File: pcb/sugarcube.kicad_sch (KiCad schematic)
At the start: 0 parts

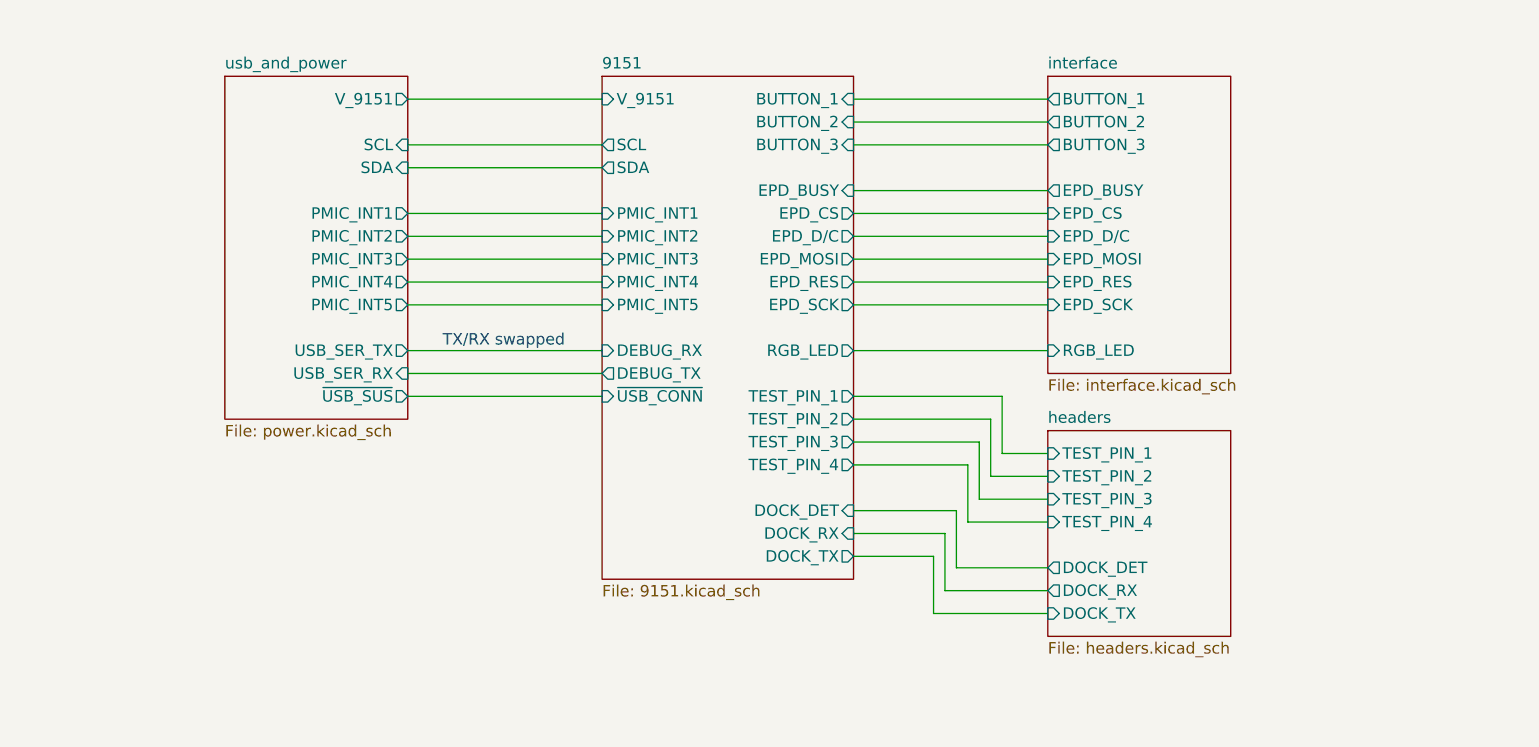
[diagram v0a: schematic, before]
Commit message: Adding filters
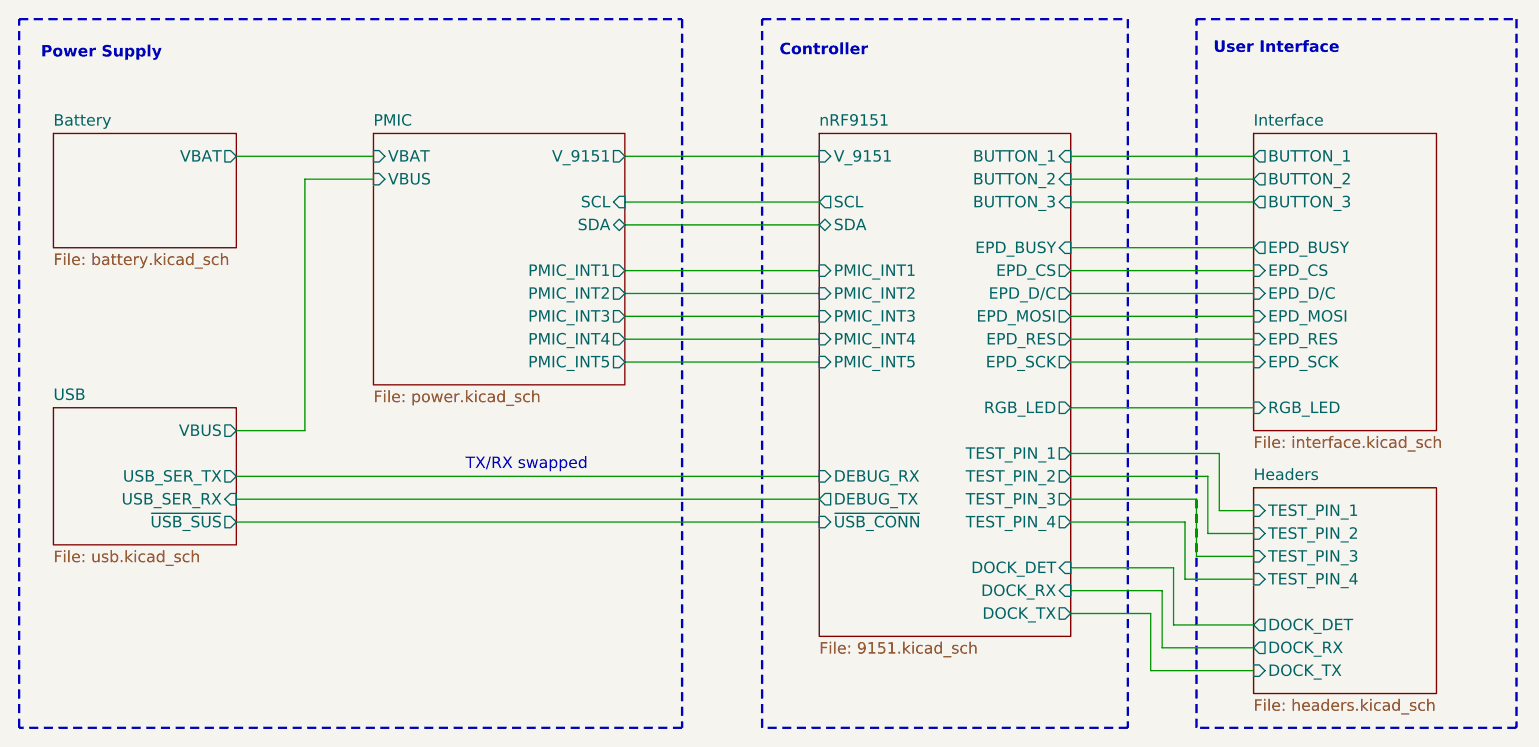
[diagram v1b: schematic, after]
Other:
- sheet 9151 renamed nRF9151
- sheet headers renamed Headers
- sheet interface renamed Interface
- sheet usb_and_power renamed PMIC
- added sheet Battery (battery.kicad_sch)
- added sheet USB (usb.kicad_sch)
- sheet PMIC ports: added VBAT, VBUS; removed USB_SER_RX, USB_SER_TX, ~{USB_SUS}
- note added: "Controller"
- note added: "Power Supply"
- note added: "User Interface"
